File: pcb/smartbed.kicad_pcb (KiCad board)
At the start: 2 copper layers, 98 x 56 mm, 53 parts, among them J1 USB_MICRO_A, J2 SBBUS_1, J3 DBGCON, J4 GPIOCON, J5 GPIOCON, J6 FSRCON1, J7 FSRCON2, J8 SBBUS_2, SW1 SW_SPST, U1 LD1117S33CTR, U2 ATSAMD21J18A, Y1 Crystal

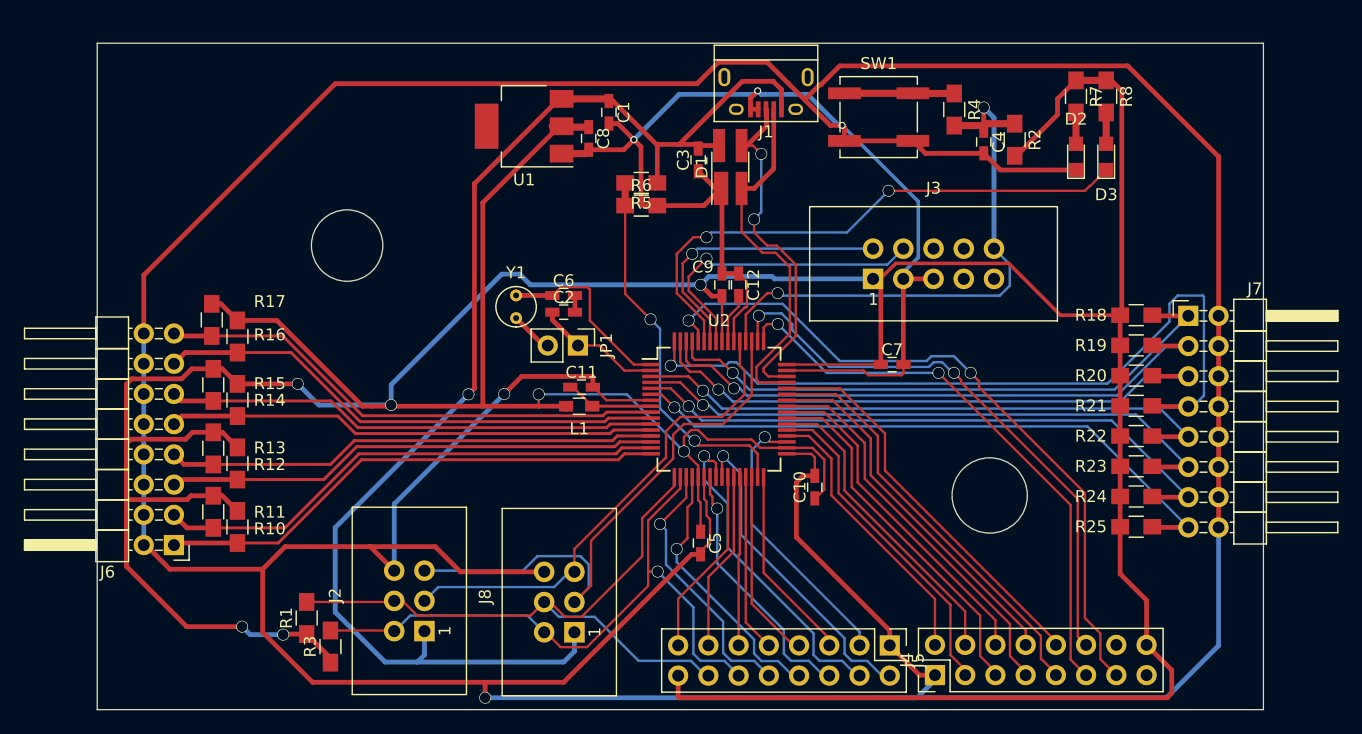
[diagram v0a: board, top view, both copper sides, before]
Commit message: Revision 2
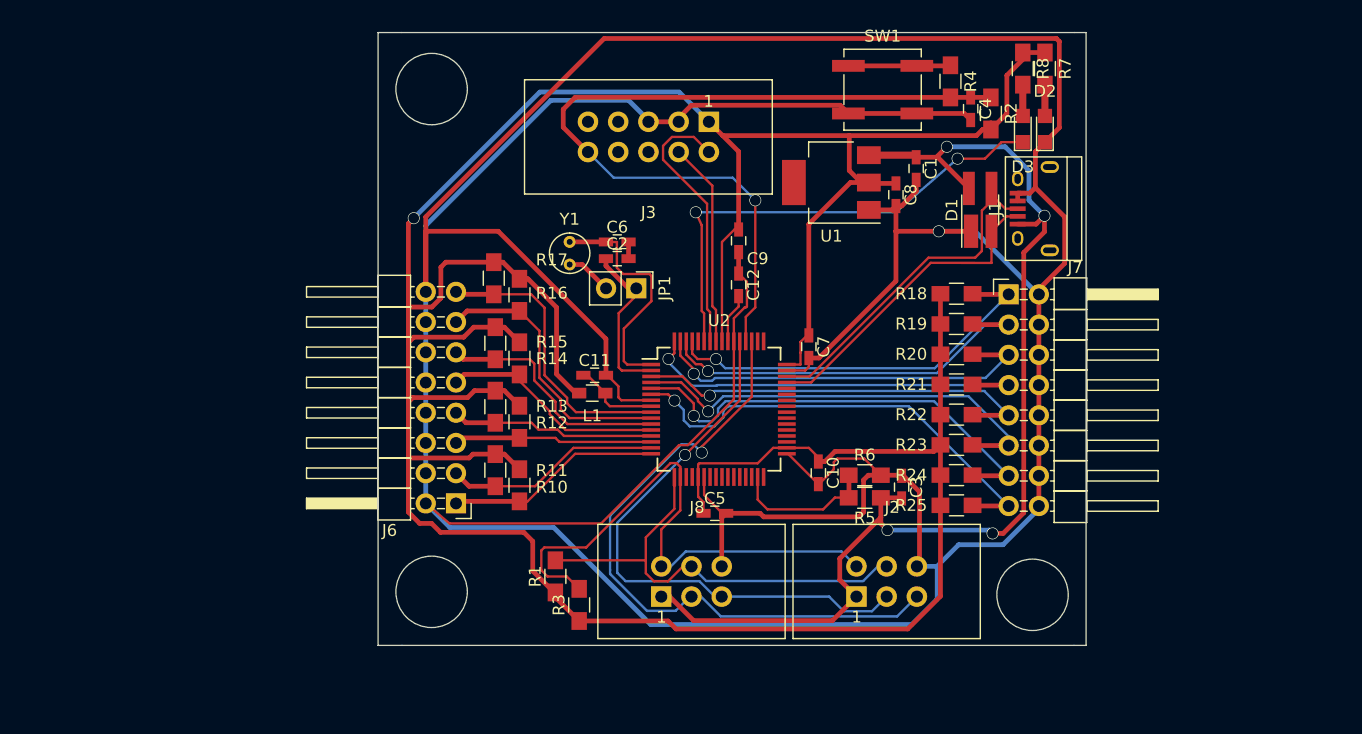
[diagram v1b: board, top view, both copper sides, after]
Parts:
- removed J4, J5: GPIOCON, Pin_Headers:Pin_Header_Straight_2x08_Pitch2.54mm
- moved J2 36.4 mm to (170.8, 93.5), turned to 0 degrees
- moved R5 32.5 mm to (171.5, 85.2)
- moved C3 32.4 mm to (174.6, 84.3), turned to 270 degrees
- moved R6 29.4 mm to (171.5, 83.3)
- moved C1 26.2 mm to (175.8, 57.5)
- moved C8 26.2 mm to (174.1, 59.7)
- moved U1 26.2 mm to (168.7, 58.7)
- moved J1 24.5 mm to (185.7, 60.9), turned to 90 degrees
- moved J6 24.0 mm to (137.2, 85.7)
- moved R10 24.0 mm to (142.5, 84.1)
- moved R11 24.0 mm to (140.5, 82.9)
- moved R12 24.0 mm to (142.5, 78.8)
- moved R13 24.0 mm to (140.5, 77.5)
- moved R14 24.0 mm to (142.5, 73.5)
- moved R15 24.0 mm to (140.5, 72.2)
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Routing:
- net GND: track 515.8 -> 413.2 mm, vias 5 -> 1
- net +3V3: track 384.2 -> 296.4 mm, vias 7 -> 1
- net PB31: track 59.6 -> 0.00 mm, vias 2 -> 0
- net PB23: track 48.8 -> 0.00 mm, vias 2 -> 0
- net PB22: track 48.2 -> 0.00 mm, vias 2 -> 0
- net PA22: track 35.4 -> 0.00 mm
- net PA23: track 33.5 -> 0.00 mm
- net PA20: track 32.9 -> 0.00 mm
- net PA21: track 31.1 -> 0.00 mm
- net PB16: track 30.6 -> 0.00 mm
- net FSR11: track 64.9 -> 34.8 mm
- net PB17: track 28.7 -> 0.00 mm
- net PA18: track 28.1 -> 0.00 mm
- net PB11: track 27.6 -> 0.00 mm, vias 1 -> 0
- net PB12: track 27.2 -> 0.00 mm, vias 1 -> 0
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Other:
- board size 98 x 56 mm -> 59.5 x 51.5 mm
